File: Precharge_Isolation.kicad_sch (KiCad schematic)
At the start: 4 parts, among them K1 DE1a-12V, Q1 NMOS

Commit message: fixed hv placement
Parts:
- R32: footprint (none) -> Resistor_SMD:R_0603_1608Metric_Pad0.98x0.95mm_HandSolder
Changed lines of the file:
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@@
 			)
 		)
-		(property "Footprint" ""
+		(property "Footprint" "Resistor_SMD:R_0603_1608Metric_Pad0.98x0.95mm_HandSolder"
 			(at 76.2 42.418 90)
 			(hide yes)

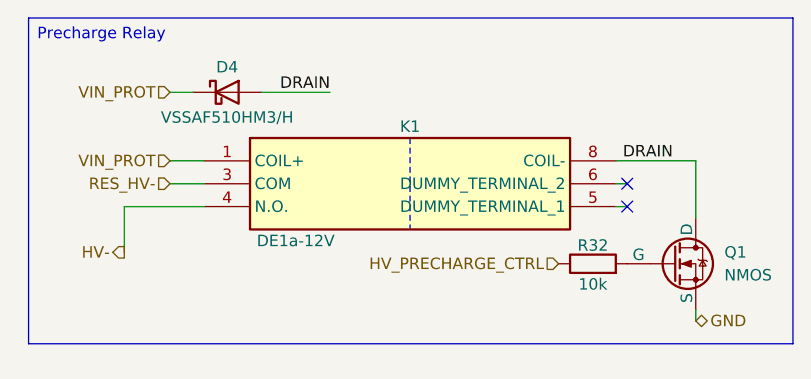
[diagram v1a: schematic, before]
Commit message: restored pp placement
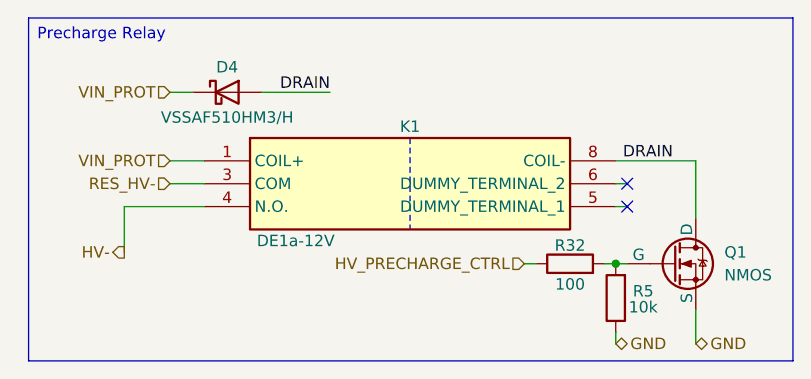
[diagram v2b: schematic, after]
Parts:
- added R5: 10k, Resistor_SMD:R_0603_1608Metric_Pad0.98x0.95mm_HandSolder, symbol Device:R
- R32: value 10k -> 100
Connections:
- net GND: now also R5.1
- net at Q1.2 (G), R32.2: now also R5.2
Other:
- moved on the sheet: R32
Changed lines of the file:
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@@
 	(rectangle
 		(start 13.4938 13.3349)
-		(end 98.4249 49.5299)
+		(end 98.4249 51.4349)
 		(stroke
 			(width 0)
@@
 		)
 	)
+	(junction
+		(at 78.74 40.64)
+		(diameter 0)
+		(color 0 0 0 0)
+	)
 	(no_connect
 		(at 80.01 31.75)
@@
 	(wire
 		(pts
+			(xy 78.74 40.64) (xy 80.01 40.64)
+		)
+		(stroke
+			(width 0)
+			(type default)
+		)
+	)
+	(wire
+		(pts
 			(xy 78.74 34.29) (xy 80.01 34.29)
 		)
@@
 		)
 	)
+	(wire
+		(pts
+			(xy 78.74 49.53) (xy 78.74 48.26)
+		)
+		(stroke
+			(width 0)
+			(type default)
+		)
+	)
+	(wire
+		(pts
+			(xy 77.47 40.64) (xy 78.74 40.64)
+		)
+		(stroke
+			(width 0)
+			(type default)
+		)
+	)
+	(wire
+		(pts
+			(xy 69.85 40.64) (xy 68.58 40.64)
+		)
+		(stroke
+			(width 0)
+			(type default)
+		)
+	)
 	(polyline
 		(pts
@@
 	(wire
 		(pts
-			(xy 87.63 46.99) (xy 87.63 45.72)
+			(xy 87.63 49.53) (xy 87.63 45.72)
 		)
 		(stroke
@@
 	(hierarchical_label "GND"
 		(shape bidirectional)
-		(at 87.63 46.99 0)
+		(at 87.63 49.53 0)
 		(effects
 			(font
@@
 	(hierarchical_label "HV_PRECHARGE_CTRL"
 		(shape input)
-		(at 72.39 40.64 180)
+		(at 68.58 40.64 180)
 		(effects
 			(font
@@
 		)
 	)
+	(hierarchical_label "GND"
+		(shape bidirectional)
+		(at 78.74 49.53 0)
+		(effects
+			(font
+				(size 1.27 1.27)
+			)
+			(justify left)
+		)
+	)
 	(hierarchical_label "RES_HV-"
 		(shape input)
@@
 			)
 			(justify right)
+		)
+	)
+	(symbol
+		(lib_id "Device:R")
+		(at 78.74 44.45 180)
+		(unit 1)
+		(body_style 1)
+		(exclude_from_sim no)
+		(in_bom yes)
+		(on_board yes)
+		(in_pos_files yes)
+		(dnp no)
+		(property "Reference" "R5"
+			(at 81.788 43.688 0)
+			(show_name no)
+			(do_not_autoplace no)
+			(effects
+				(font
+					(size 1.27 1.27)
+				)
+			)
+		)
+		(property "Value" "10k"
+			(at 81.788 45.466 0)
+			(show_name no)
+			(do_not_autoplace no)
+			(effects
+				(font
+					(size 1.27 1.27)
+				)
+			)
+		)
+		(property "Footprint" "Resistor_SMD:R_0603_1608Metric_Pad0.98x0.95mm_HandSolder"
+			(at 80.518 44.45 90)
+			(hide yes)
+			(show_name no)
+			(do_not_autoplace no)
+			(effects
+				(font
+					(size 1.27 1.27)
+				)
+			)
+		)
+		(property "Datasheet" ""
+			(at 78.74 44.45 0)
+			(hide yes)
+			(show_name no)
+			(do_not_autoplace no)
+			(effects
+				(font
+					(size 1.27 1.27)
+				)
+			)
+		)
+		(property "Description" "Resistor"
+			(at 78.74 44.45 0)
+			(hide yes)
+			(show_name no)
+			(do_not_autoplace no)
+			(effects
+				(font
+					(size 1.27 1.27)
+				)
+			)
+		)
+		(pin "2"
+		)
+		(pin "1"
+		)
+		(instances
+			(project "PS-PrechargeBoard"
+				(path "/74d17fe6-68d4-4bd7-954a-e2bbb58b1f1e/5b236d54-dfec-450f-96e4-88b51678f51f"
+					(reference "R36")
+					(unit 1)
+				)
+				(path "/74d17fe6-68d4-4bd7-954a-e2bbb58b1f1e/d5231689-0a25-4774-9952-2a5e507de834"
+					(reference "R5")
+					(unit 1)
+				)
+			)
 		)
 	)
@@
 	(symbol
 		(lib_id "Device:R")
-		(at 76.2 40.64 90)
+		(at 73.66 40.64 90)
 		(unit 1)
 		(body_style 1)
@@
 		(dnp no)
 		(property "Reference" "R32"
-			(at 76.2 38.608 90)
-			(show_name no)
-			(do_not_autoplace no)
-			(effects
-				(font
-					(size 1.27 1.27)
-				)
-			)
-		)
-		(property "Value" "10k"
-			(at 76.2 42.926 90)
+			(at 73.66 38.608 90)
+			(show_name no)
+			(do_not_autoplace no)
+			(effects
+				(font
+					(size 1.27 1.27)
+				)
+			)
+		)
+		(property "Value" "100"
+			(at 73.66 42.926 90)
 			(show_name no)
 			(do_not_autoplace no)
@@
 		)
 		(property "Footprint" "Resistor_SMD:R_0603_1608Metric_Pad0.98x0.95mm_HandSolder"
-			(at 76.2 42.418 90)
+			(at 73.66 42.418 90)
 			(hide yes)
 			(show_name no)
@@
 		)
 		(property "Datasheet" ""
-			(at 76.2 40.64 0)
+			(at 73.66 40.64 0)
 			(hide yes)
 			(show_name no)
@@
 		)
 		(property "Description" "Resistor"
-			(at 76.2 40.64 0)
-			(hide yes)
-			(show_name no)
+			(at 73.66 40.64 0)
+			(hide yes)
+			(show_name no)
